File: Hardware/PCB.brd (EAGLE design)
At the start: 46 x 35 mm, 105 parts, among them IC1 BQ25180YBGR_BQ25180YBGR, IC2 DRV2605YZFR_DRV2605YZFR, IC3 BMA423_BMA423, IC9 RT6160AWSC_RT6160AWSC, J1 503480-2400_503480-2400, J2 TC2030-IDC_TC2030-IDC, J4 KH-TYPE-C-16P_KH-TYPE-C-16P, Q1 20V/4.2A/52mΩ/1.4W, Q3 SI1308EDL-T1-GE3, U1 NORDIC_NRF_4_NRF52840_QF, U3 ESP32_C6_LIBRARY_MAX17048G+T10, X1 32MHz, X2 32.768kHz

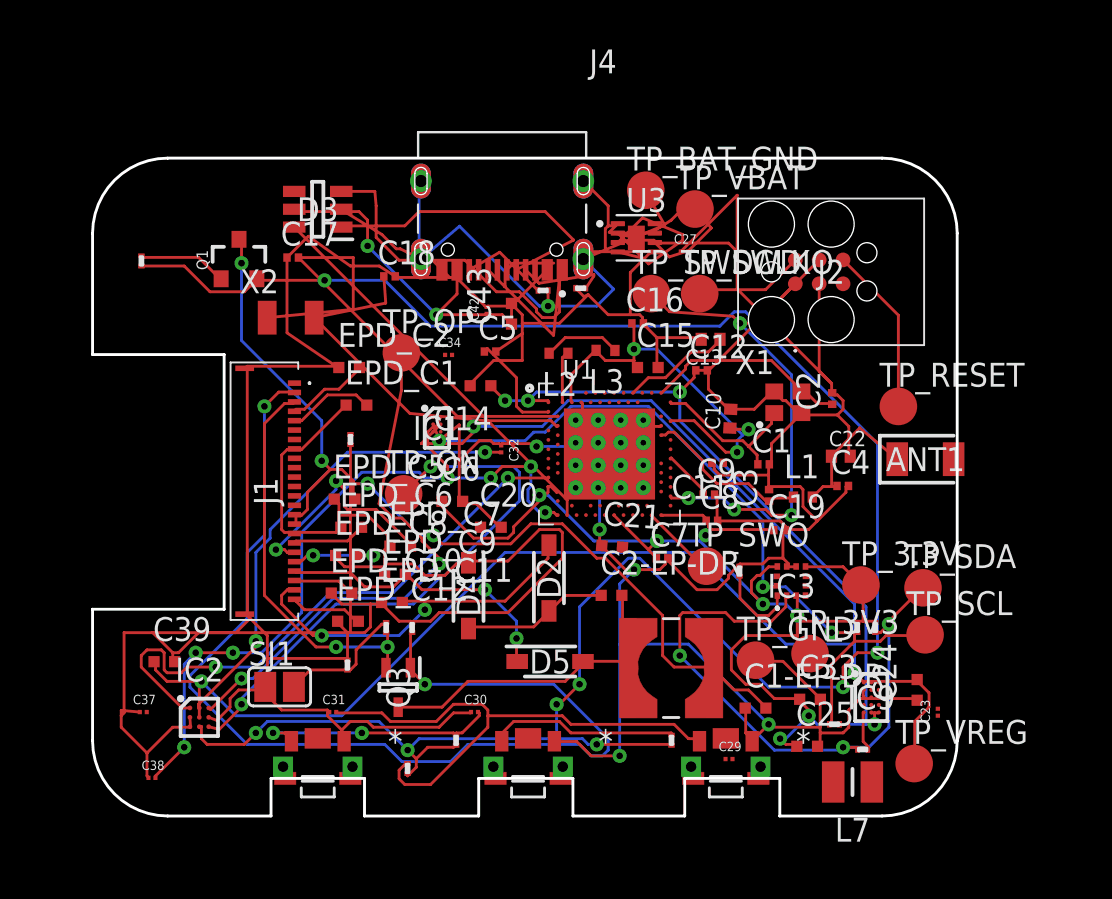
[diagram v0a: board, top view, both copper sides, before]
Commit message: Update repository
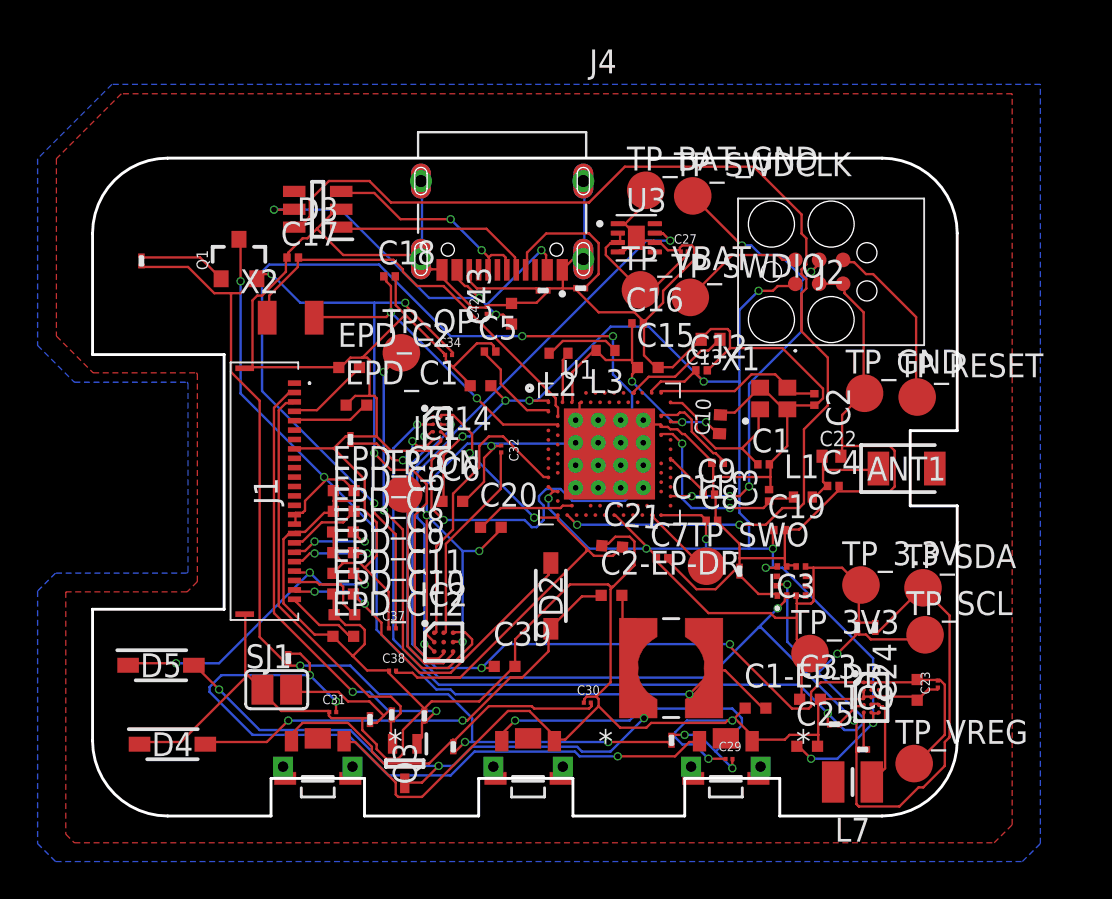
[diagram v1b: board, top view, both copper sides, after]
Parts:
- moved D5 20.7 mm to (3.64, 8.02)
- moved C39 18.1 mm to (21.9, 7.96)
- moved D4 17.6 mm to (4.25, 3.82), turned to 0 degrees
- moved TP_GND 15.3 mm to (41.1, 22.5)
- moved C38 14.0 mm to (16.0, 7.73)
- moved C37 14.0 mm to (15.9, 9.98)
- moved IC2 13.6 mm to (18.7, 9.25)
- moved R8 8.63 mm to (10.4, 8.38)
- moved C30 6.02 mm to (26.3, 6.03)
- moved TP_SWDCLK 5.65 mm to (31.9, 33.0)
- moved TP_VBAT 5.19 mm to (29.1, 28.0)
- moved R2_EP_DR 4.74 mm to (17.6, 5.33)
- moved R1_EP_DR 4.66 mm to (15.9, 5.38)
- moved Q3 4.07 mm to (16.6, 2.79)
- moved EPD_C7 3.14 mm to (13.3, 15.1)
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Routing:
- net VBAT/2.5C: track 0.00 -> 69.2 mm, vias 0 -> 4
- net D-: track 21.3 -> 61.0 mm, vias 0 -> 2
- net VREG: track 86.8 -> 50.8 mm
- net GND: track 404.0 -> 368.4 mm
- net SDA/2.4C: track 32.6 -> 65.9 mm
- net GDR: track 57.8 -> 25.5 mm
- net SCL/1.4C: track 0.00 -> 29.6 mm, vias 0 -> 2
- net 3V3/1.7D: track 115.9 -> 87.2 mm, vias 8 -> 6
- net N$72: track 17.5 -> 36.6 mm, vias 0 -> 3
- net OUT-: track 30.3 -> 11.3 mm, vias 2 -> 0
- net DP: track 29.4 -> 11.7 mm, vias 0 -> 2
- net N$81: track 7.79 -> 25.1 mm, vias 0 -> 2
- net SCL/2.4C: track 41.0 -> 57.1 mm, vias 3 -> 4
- net HAPTIC_EN: track 31.2 -> 15.8 mm, vias 2 -> 0
- net N$71: track 25.1 -> 10.9 mm, vias 2 -> 0
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- added copper zone on layer 1, net GND
- added copper zone on layer 16, net GND
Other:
- outline, holes or cut-outs redrawn
